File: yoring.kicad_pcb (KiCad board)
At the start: 4 copper layers, 31.1 x 50 mm, 71 parts, among them J1 USB-C_USB4105-GF-A, J3 Conn_01x05, SW1 SW_MEC_5E, SW2 SW_MEC_5E, U1 ESP32C3, U2 IS25LP016D-JLLE, U3 USBLC6-2SC6, U4 ICM-20602, U5 ICM-20602, U6 ICM-20602, U7 AMS1117-3.3, U8 USBLC6-2SC6, Y1 40.000MHZ

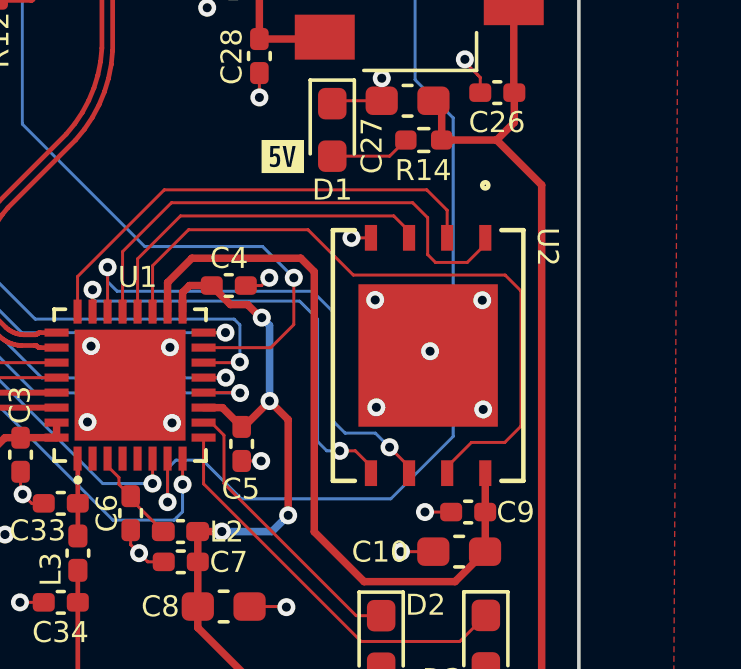
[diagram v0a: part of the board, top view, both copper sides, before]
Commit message: Commit before local repo deletion
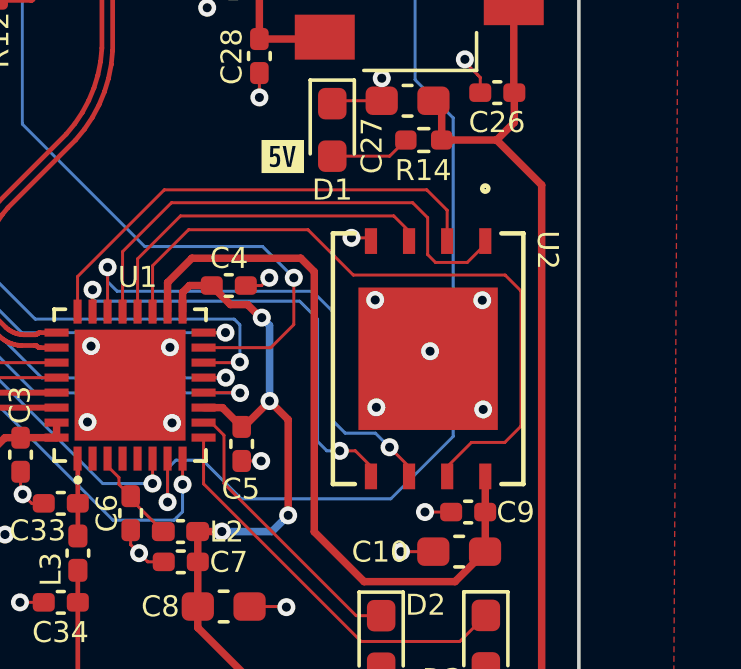
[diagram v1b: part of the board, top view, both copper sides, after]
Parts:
- moved U2 0.11 mm to (120.3, 66.5)
